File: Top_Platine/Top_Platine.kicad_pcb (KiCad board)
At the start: 2 copper layers, 116.4 x 99.9 mm, 15 parts, among them SW1 SW_SPST, SW2 SW_SPST, SW3 SW_SPST, U2 Main Conector to Main pcb

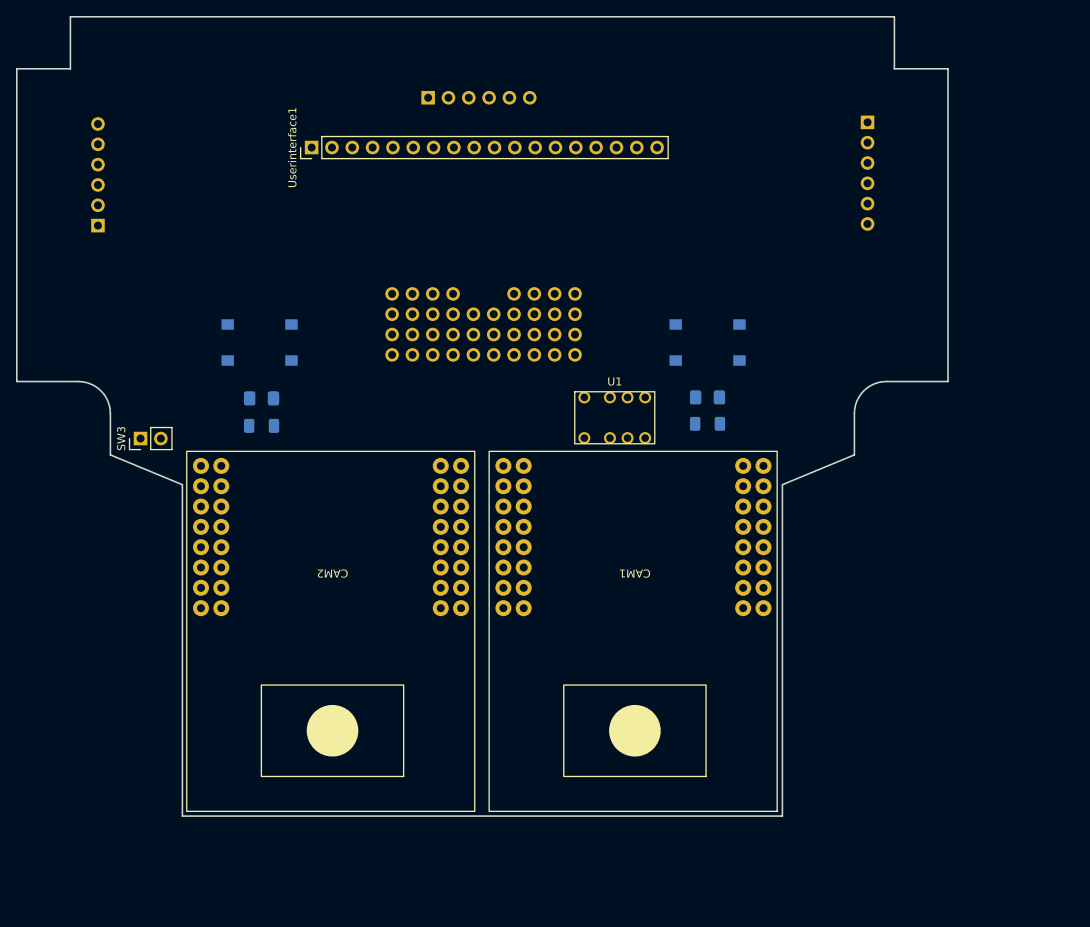
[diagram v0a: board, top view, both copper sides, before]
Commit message: add main PCB
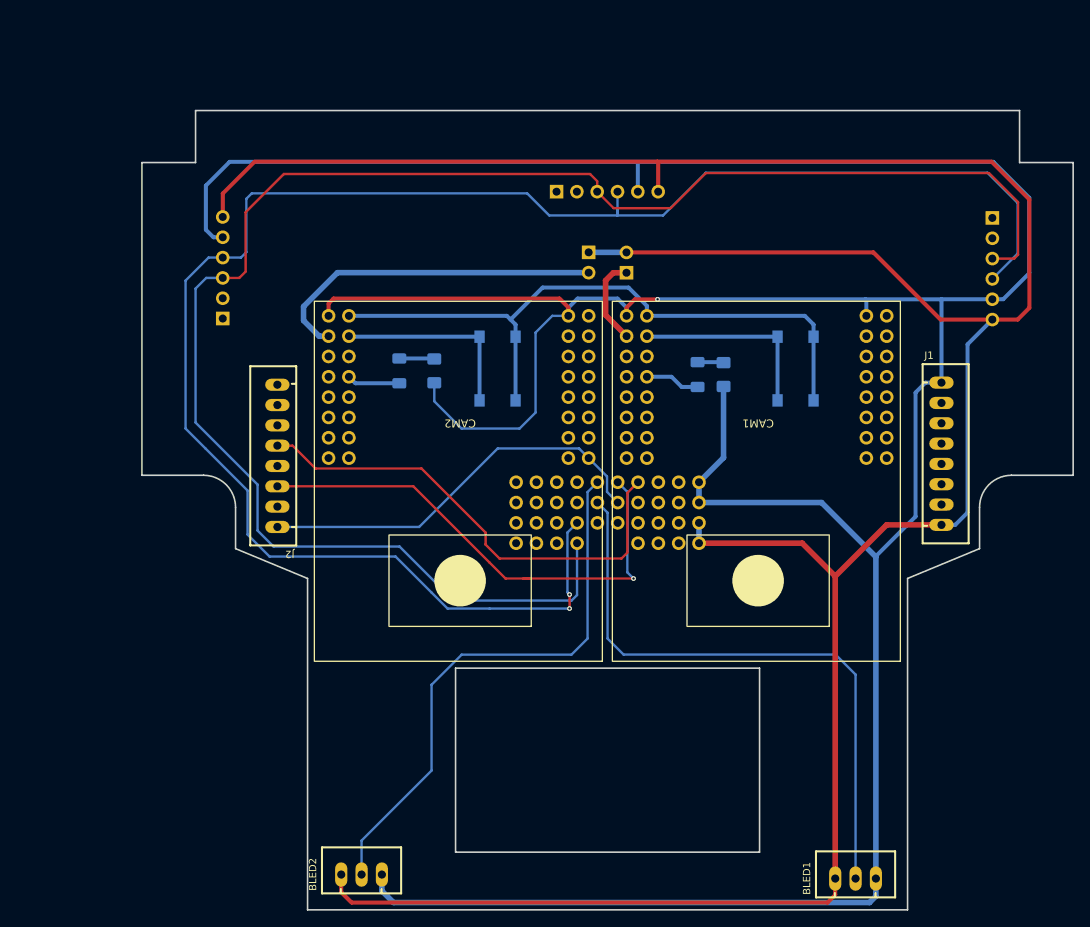
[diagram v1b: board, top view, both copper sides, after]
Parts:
- removed SW3: SW_SPST, Connector_PinHeader_2.54mm:PinHeader_1x02_P2.54mm_Vertical
- removed U1: ~, Robotik:Untitled
- removed Userinterface1: Conn_01x18_Pin, Connector_PinHeader_2.54mm:PinHeader_1x18_P2.54mm_Vertical
- added BLED1: Conn_01x03_Pin, JST:JST-XH-03-PACKAGE-LONG-PAD, F.Cu at (187.5, 147.0)
- added BLED2: Conn_01x03_Pin, JST:JST-XH-03-PACKAGE-LONG-PAD, F.Cu at (125.8, 146.5)
- added J1: Conn_01x08_Pin, JST:JST-XH-08-PACKAGE-LONG-PAD, F.Cu at (198.2, 93.9)
- added J2: Conn_01x08_Pin, JST:JST-XH-08-PACKAGE-LONG-PAD, F.Cu at (115.2, 94.2)
- added SWC1: SW_SPST, Connector_PinHeader_2.54mm:PinHeader_1x02_P2.54mm_Horizontal, B.Cu at (158.9, 71.3)
- added SWC2: SW_SPST, Connector_PinHeader_2.54mm:PinHeader_1x02_P2.54mm_Horizontal, B.Cu at (154.1, 68.7)
- moved ToF_Vorne_1 111.8 mm to (204.6, 64.4), turned to 180 degrees
- moved ToF_Vorne_2 39.8 mm to (150.1, 61.1), turned to -90 degrees
- moved ToF_Vorne_3 37.7 mm to (108.4, 77.0), turned to 0 degrees
- moved SW2 29.9 mm to (142.8, 83.2), turned to 90 degrees
- moved U2 24.7 mm to (155.2, 100.0), turned to 0 degrees
- moved CAM2 24.6 mm to (155.8, 74.8)
- moved CAM1 24.3 mm to (193.1, 74.8)
- moved D2 21.9 mm to (134.8, 83.5), turned to 90 degrees
- moved RV2 18.5 mm to (130.5, 83.5), turned to 90 degrees
- moved SW1 11.5 mm to (180.0, 83.2), turned to 90 degrees
- moved RV1 6.29 mm to (167.8, 84.0), turned to 90 degrees
- moved D1 3.49 mm to (171.0, 84.0), turned to 90 degrees
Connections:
- CAM1 pad 17: unconnected-(CAM1-3.3V-Pad17) -> +3.3V
- CAM1 pad 26: /Kamera/PWR_CAM1 -> /Kamera/Kamera1/5V
- CAM1 pad 29: unconnected-(CAM1-P9-Pad29) -> /INTT_C1
- CAM1 pad 30: unconnected-(CAM1-P10-Pad30) -> /INT_C1
- CAM1 pad 32: /RST_C1 -> unconnected-(CAM1-RST-Pad32)
- CAM1 pad 5: /Kamera/SCK -> /Kamera/Kamera1/SS
- CAM1 pad 6: /CS_C1 -> /Kamera/Kamera1/SCLK
- CAM1 pad 7: /Kamera/MISO -> /Kamera/Kamera1/MISO
- CAM1 pad 8: /Kamera/MOSI -> /Kamera/Kamera1/MOSI
- CAM2 pad 17: unconnected-(CAM2-3.3V-Pad17) -> +3.3V
- CAM2 pad 26: /Kamera/PWR_CAM2 -> /Kamera/Kamera2/5V
- CAM2 pad 29: unconnected-(CAM2-P9-Pad29) -> /INTT_C2
- CAM2 pad 30: unconnected-(CAM2-P10-Pad30) -> /INT_C2
- CAM2 pad 32: /RST_C2 -> unconnected-(CAM2-RST-Pad32)
- CAM2 pad 5: /Kamera/SCK -> /Kamera/Kamera2/SS
- CAM2 pad 6: /CS_C2 -> /Kamera/Kamera2/SCLK
- CAM2 pad 7: /Kamera/MISO -> /Kamera/Kamera2/MISO
- CAM2 pad 8: /Kamera/MOSI -> /Kamera/Kamera2/MOSI
- U2 pad CS_C1: unconnected-(U2-Chip_Select_Cam_1-PadCS_C1) -> /CS_C1
- U2 pad CS_C2: unconnected-(U2-Chip_Select_Cam_2-PadCS_C2) -> /CS_C2
- U2 pad CS_D: unconnected-(U2-CS_Display-PadCS_D) -> /CS_D
- U2 pad D_D: unconnected-(U2-D_Display-PadD_D) -> /D_D
- U2 pad I_C1: unconnected-(U2-Interrupt_Cam_1-PadI_C1) -> /INT_C1
- U2 pad I_C2: unconnected-(U2-Interrupt_Cam_2-PadI_C2) -> /INT_C2
- U2 pad LED1: unconnected-(U2-Beleuchtung_Cam_1-PadLED1) -> /BLED_C1
- U2 pad LED2: unconnected-(U2-Beleuchtung_Cam_2-PadLED2) -> /BLED_C2
- U2 pad MOSI: unconnected-(U2-PadMOSI) -> /MOSI
- U2 pad RX_C1: unconnected-(U2-RX_Cam_1-PadRX_C1) -> /RX_C1
- U2 pad RX_C2: unconnected-(U2-RX_Cam_2-PadRX_C2) -> /RX_C2
- U2 pad R_C1: unconnected-(U2-Reset_Cam_1-PadR_C1) -> /INTT_C1
- U2 pad R_C2: unconnected-(U2-Reset_Cam_2-PadR_C2) -> /INTT_C2
- U2 pad SCK: unconnected-(U2-PadSCK) -> /SCK
- U2 pad TX_C1: unconnected-(U2-TX_Cam_1-PadTX_C1) -> /TX_C1
- U2 pad TX_C2: unconnected-(U2-TX_Cam_2-PadTX_C2) -> /TX_C2
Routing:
- net GND: track 0.00 -> 442.8 mm, vias 0 -> 1
- net +5V: track 0.00 -> 355.1 mm
- net /SDA: track 0.00 -> 222.0 mm, vias 0 -> 2
- net /SCL: track 0.00 -> 212.7 mm
- net +3.3V: track 0.00 -> 84.0 mm
- net /RX_C1: track 0.00 -> 78.0 mm
- net /BLED_C1: track 0.00 -> 75.9 mm
- net /ToF_XS_1: track 0.00 -> 72.6 mm
- net /BLED_C2: track 0.00 -> 69.3 mm
- net /TX_C1: track 0.00 -> 67.6 mm
- net /RE_A: track 0.00 -> 64.1 mm
- net /D_D: track 0.00 -> 62.9 mm, vias 0 -> 1
- net /RE_B: track 0.00 -> 60.3 mm
- net /CS_D: track 0.00 -> 60.1 mm
- net /ToF_XS_3: track 0.00 -> 59.8 mm
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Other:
- outline, holes or cut-outs redrawn
- copper layers 2 -> 4
